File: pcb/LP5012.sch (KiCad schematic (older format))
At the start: 14 parts, among them J1 Main Connector, U1 LP5012

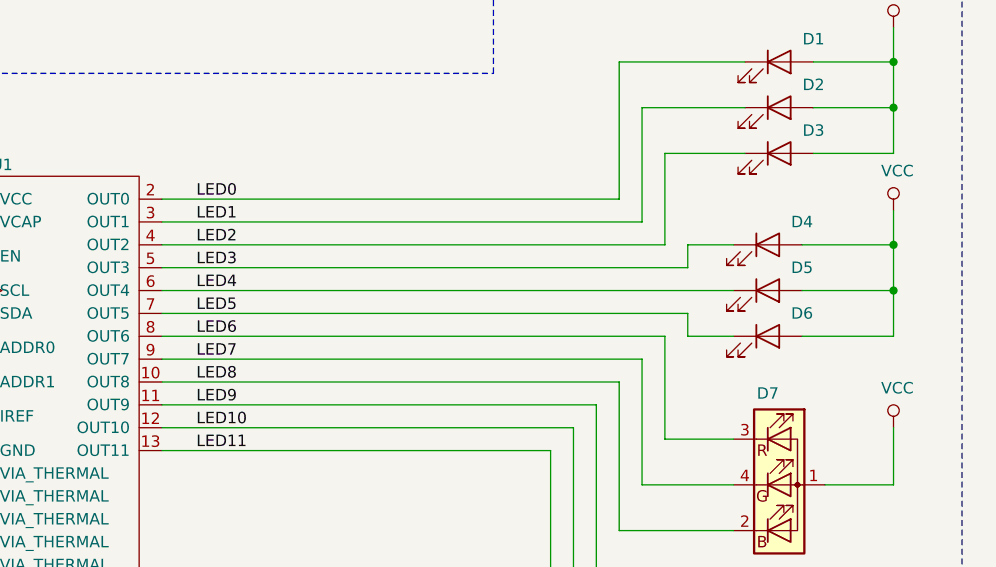
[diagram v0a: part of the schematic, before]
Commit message: Ultimas modificaciones
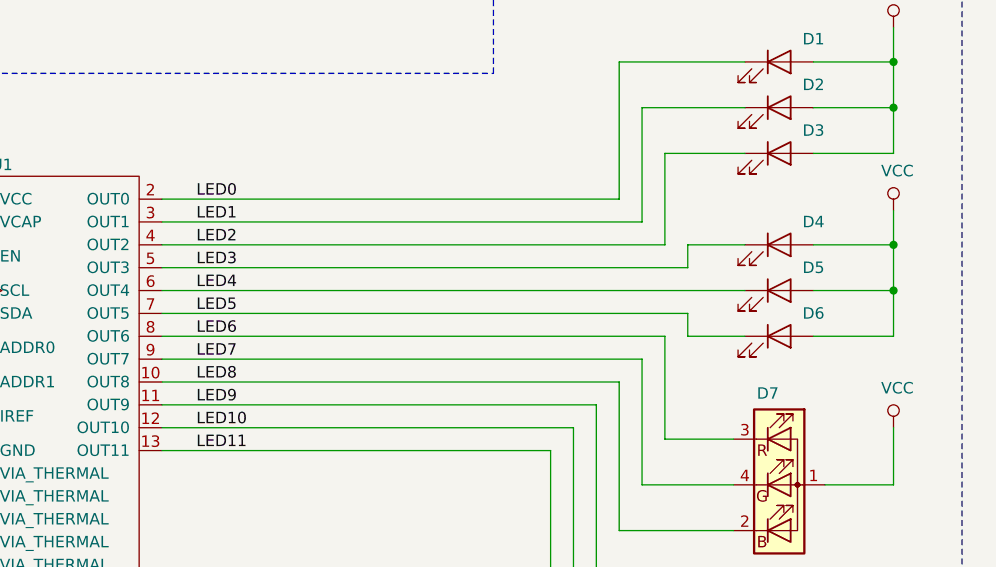
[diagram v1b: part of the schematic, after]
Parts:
- C2, C3: Link (none) -> https://ar.mouser.com/ProductDetail/KEMET/C0805C105K3RACTU?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; SKU (none) -> 80-C0805C105K3R; Supplier (none) -> Mouser
- C4: Link (none) -> https://ar.mouser.com/ProductDetail/KEMET/C0805C104J5RACTU?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; SKU (none) -> 80-C0805C104J5R; Supplier (none) -> Mouser
- D1, D2, D3, D4, D5, D6: Link (none) -> https://ar.mouser.com/ProductDetail/Inolux/IN-S85ATG?qs=sGA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; SKU (none) -> 743-IN-S85ATG; Supplier (none) -> Mouser
- D7, D8: Link (none) -> 638-19237R6GHBHCA01; SKU (none) -> 638-19237R6GHBHCA01; Supplier (none) -> Mouser
- R4: Link (none) -> https://ar.mouser.com/ProductDetail/Vishay-Dale/CRCW08053K3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; SKU (none) -> 71-CRCW08053K30FKEAC; Supplier (none) -> Mouser
- U1: Link (none) -> https://ar.mouser.com/ProductDetail/Texas-Instruments/LP501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; SKU (none) -> 595-LP5012RUKR; Supplier (none) -> Mouser
